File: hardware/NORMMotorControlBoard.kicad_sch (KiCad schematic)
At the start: 18 parts, among them J1 Back Left Motor, J2 Front Left Motor, J3 Front Right Motor, J4 Back Right Motor, J5 USB4125-GF-A_REVA2, J6 Conn_01x04_Pin, M1 Front Motors, M2 Back Motors, SW1 Reset, U1 SN74LVC2G14DBV, U2 SN74LVC2G14DBV

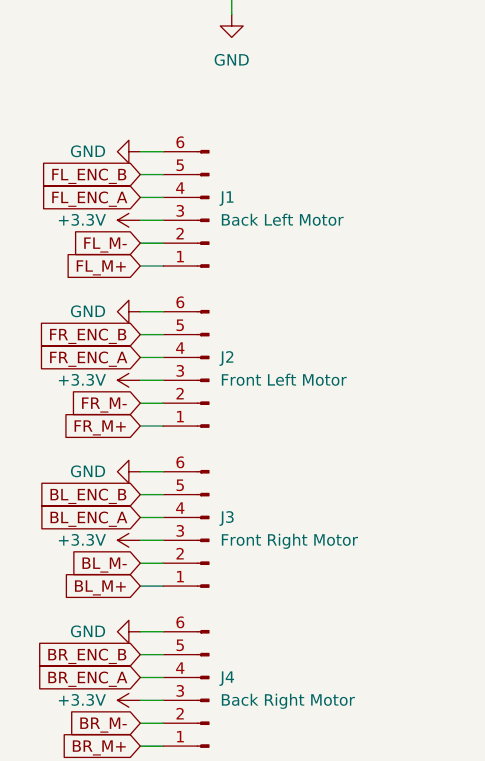
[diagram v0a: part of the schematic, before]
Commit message: Exported board v1.1
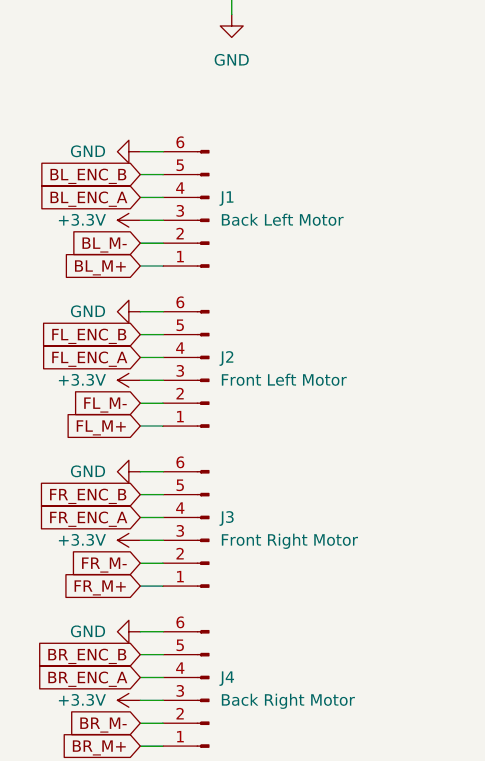
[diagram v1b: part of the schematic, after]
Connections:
- net BL_ENC_A: now also J1.4 (Pin_4); no longer J3.4 (Pin_4)
- net BL_ENC_B: now also J1.5 (Pin_5); no longer J3.5 (Pin_5)
- net BL_M+: now also J1.1 (Pin_1); no longer J3.1 (Pin_1)
- net BL_M-: now also J1.2 (Pin_2); no longer J3.2 (Pin_2)
- net FL_ENC_A: now also J2.4 (Pin_4); no longer J1.4 (Pin_4)
- net FL_ENC_B: now also J2.5 (Pin_5); no longer J1.5 (Pin_5)
- net FL_M+: now also J2.1 (Pin_1); no longer J1.1 (Pin_1)
- net FL_M-: now also J2.2 (Pin_2); no longer J1.2 (Pin_2)
- net FR_ENC_A: now also J3.4 (Pin_4); no longer J2.4 (Pin_4)
- net FR_ENC_B: now also J3.5 (Pin_5); no longer J2.5 (Pin_5)
- net FR_M+: now also J3.1 (Pin_1); no longer J2.1 (Pin_1)
- net FR_M-: now also J3.2 (Pin_2); no longer J2.2 (Pin_2)

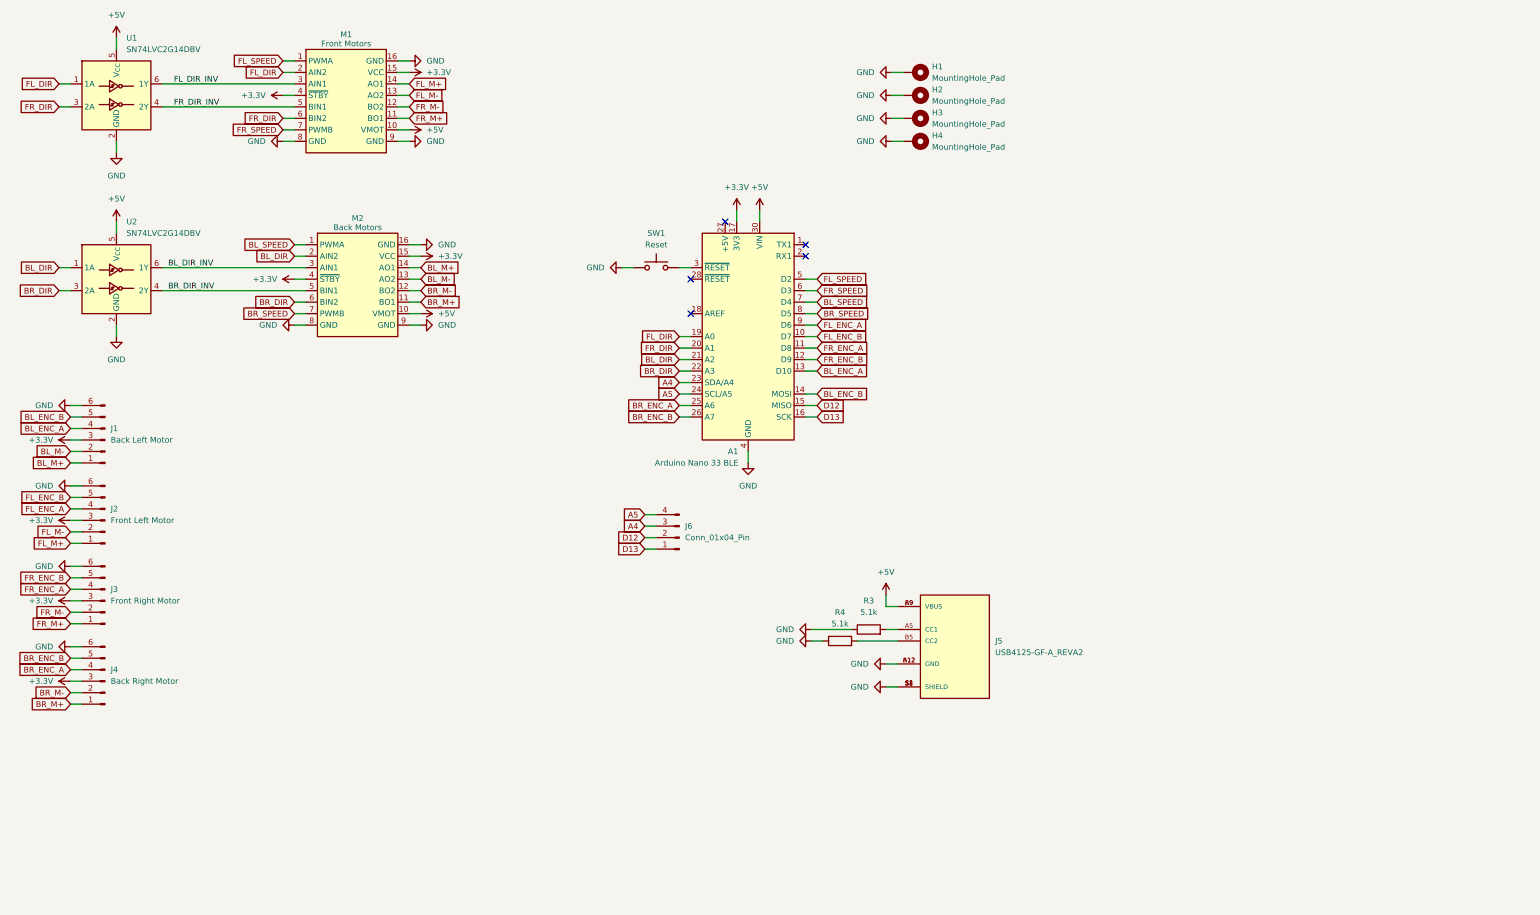
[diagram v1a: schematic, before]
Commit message: Finished schematic for V1.3
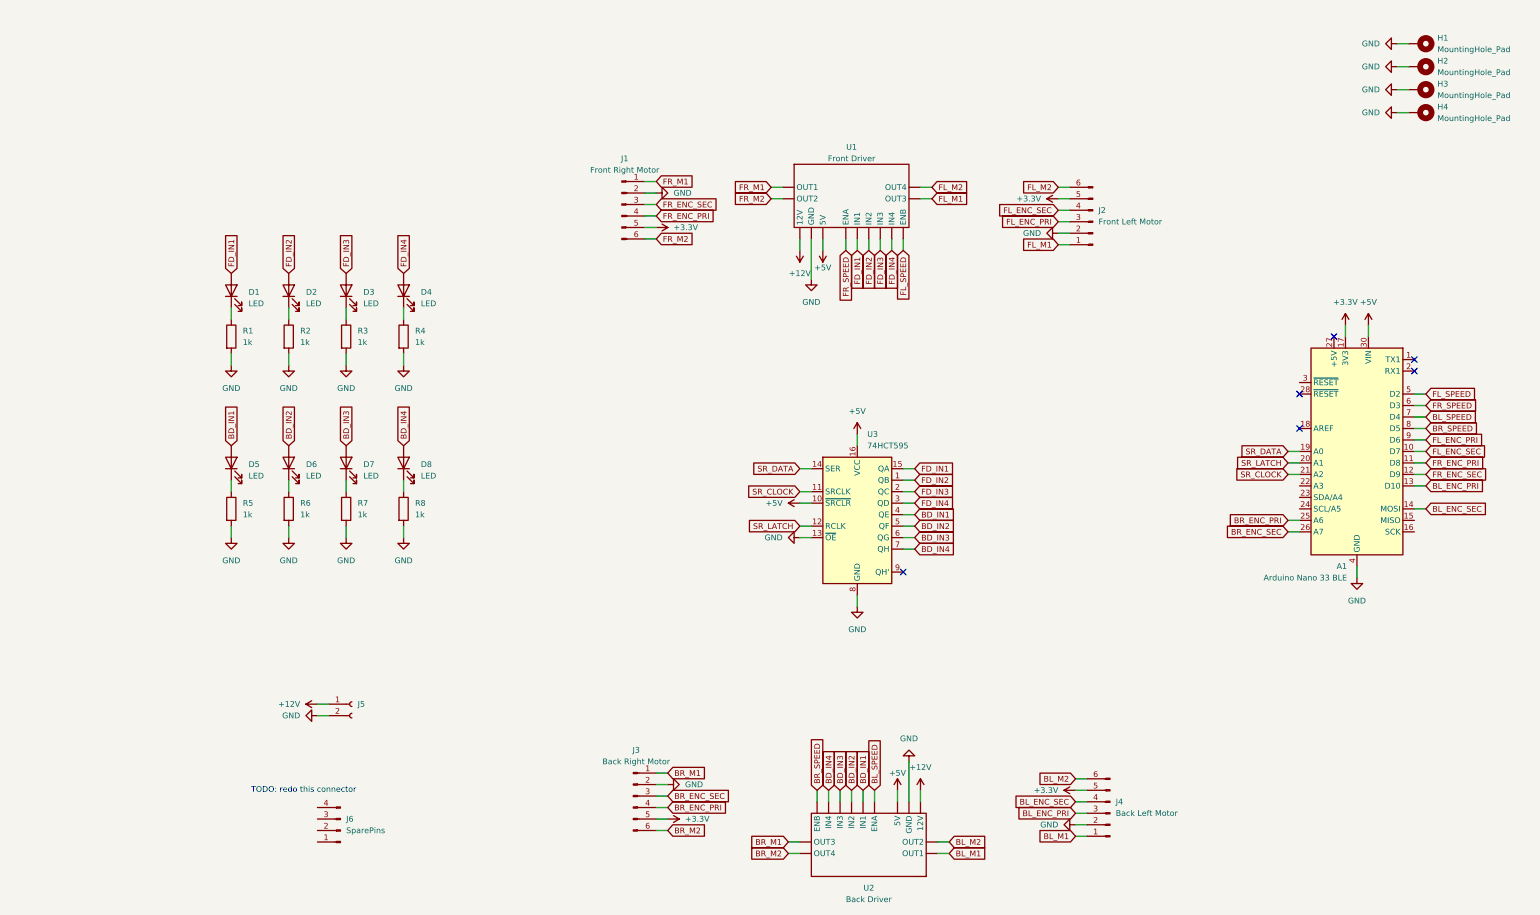
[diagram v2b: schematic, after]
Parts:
- removed J5: USB4125-GF-A_REVA2, USB_C:USB_C, symbol USB_C:USB4125-GF-A_REVA2
- removed M1: Front Motors, Pololu_MD08A_Motor_Driver:Pololu_MD08A_Motor_Driver, symbol Pololu_MD08A_Motor_Driver:Pololu_MD08A_Motor_Driver
- removed M2: Back Motors, Pololu_MD08A_Motor_Driver:Pololu_MD08A_Motor_Driver, symbol Pololu_MD08A_Motor_Driver:Pololu_MD08A_Motor_Driver
- removed SW1: Reset, Two_Pin_Through_Hole_Push_Button:Two_Pin_Through_Hole_Push_Button, symbol Switch:SW_Push
- removed U1, U2: SN74LVC2G14DBV, Package_TO_SOT_SMD:SOT-23-6, symbol 74xGxx:SN74LVC2G14DBV
- added D1, D2, D3, D4, D5, D6, D7, D8: LED, LED_SMD:LED_0603_1608Metric, symbol Device:LED
- added J5: Conn_01x02_Socket, Connector_Samtec_HPM_THT:Samtec_HPM-02-01-x-S_Straight_1x02_Pitch5.08mm, symbol Connector:Conn_01x02_Socket
- added R1, R2, R5, R6, R7, R8: 1k, Resistor_SMD:R_0603_1608Metric, symbol Device:R
- added U1: Front Driver, symbol L298N:L298N
- added U2: Back Driver, symbol L298N:L298N
- added U3: 74HCT595, Package_SO:SOIC-16_3.9x9.9mm_P1.27mm, symbol 74xx:74HCT595
- J1: value Back Left Motor -> Front Right Motor; footprint Connector_PinHeader_2.54mm:PinHeader_1x06_P2.54mm_Horizontal -> Connector_JST:JST_PH_S6B-PH-K_1x06_P2.00mm_Horizontal
- J2: footprint Connector_PinHeader_2.54mm:PinHeader_1x06_P2.54mm_Horizontal -> Connector_JST:JST_PH_S6B-PH-K_1x06_P2.00mm_Horizontal
- J3: value Front Right Motor -> Back Right Motor; footprint Connector_PinHeader_2.54mm:PinHeader_1x06_P2.54mm_Horizontal -> Connector_JST:JST_PH_S6B-PH-K_1x06_P2.00mm_Horizontal
- J4: value Back Right Motor -> Back Left Motor; footprint Connector_PinHeader_2.54mm:PinHeader_1x06_P2.54mm_Horizontal -> Connector_JST:JST_PH_S6B-PH-K_1x06_P2.00mm_Horizontal
- J6: value Conn_01x04_Pin -> SparePins
- R3, R4: value 5.1k -> 1k; footprint Resistor_SMD:R_0603_1608Metric_Pad0.98x0.95mm_HandSolder -> Resistor_SMD:R_0603_1608Metric
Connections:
- net BL_M- is gone; now on net GND: J1.2 (Pin_2)
- net BR_M- is gone; now on net GND: J4.2 (Pin_2)
- net FL_M- is gone; now on net GND: J2.2 (Pin_2)
- net FR_M- is gone; now on net GND: J3.2 (Pin_2)
- net +3.3V: now also J1.5 (Pin_5), J2.5 (Pin_5), J3.5 (Pin_5), J4.5 (Pin_5); no longer J1.3 (Pin_3), J2.3 (Pin_3), J3.3 (Pin_3), J4.3 (Pin_3)
- net +5V: now also U1. (OUT4), U2. (OUT4), U3.10 (~{SRCLR}), U3.16 (VCC)
- net BL_SPEED: now also U2. (OUT4)
- net BR_SPEED: now also U2. (OUT4)
- net FL_SPEED: now also U1. (OUT4)
- net FR_SPEED: now also U1. (OUT4)
- net GND: now also R3.2, R4.2, J5.2 (Pin_2), R1.2, R2.2, R5.2, R6.2, R7.2, R8.2, U1. (OUT4), U2. (OUT4), U3.13 (~{OE}), U3.8 (GND); no longer J1.6 (Pin_6), J2.6 (Pin_6), J3.6 (Pin_6), J4.6 (Pin_6), R3.1, R4.1
- net A4: no longer names the net of A1.23 (SDA/A4)
- net A4: no longer J6.3 (Pin_3)
- net A5: no longer names the net of A1.24 (SCL/A5)
- net A5: no longer J6.4 (Pin_4)
- net BL_DIR renamed SR_CLOCK
- net SR_CLOCK: now also U3.11 (SRCLK)
- net BL_ENC_A renamed BL_ENC_PRI
- net BL_ENC_PRI: now also J4.3 (Pin_3); no longer J1.4 (Pin_4)
- net BL_ENC_B renamed BL_ENC_SEC
- net BL_ENC_SEC: now also J4.4 (Pin_4); no longer J1.5 (Pin_5)
- net BL_M+ renamed FR_M1
- net FR_M1: now also U1. (OUT4)
- net BR_DIR: no longer names the net of A1.22 (A3)
- net BR_ENC_A renamed BR_ENC_PRI
- net BR_ENC_PRI: now also J3.4 (Pin_4); no longer J4.4 (Pin_4)
- net BR_ENC_B renamed BR_ENC_SEC
- net BR_ENC_SEC: now also J3.3 (Pin_3); no longer J4.5 (Pin_5)
- net BR_M+ renamed BL_M1
- net BL_M1: now also U2. (OUT4)
- net D12: no longer names the net of A1.15 (MISO)
- net D12: no longer J6.2 (Pin_2)
- net D13: no longer names the net of A1.16 (SCK)
- net D13: no longer J6.1 (Pin_1)
- net FL_DIR renamed SR_DATA
- net SR_DATA: now also U3.14 (SER)
- net FL_ENC_A renamed FL_ENC_PRI
- net FL_ENC_PRI: now also J2.3 (Pin_3); no longer J2.4 (Pin_4)
- net FL_ENC_B renamed FL_ENC_SEC
- net FL_ENC_SEC: now also J2.4 (Pin_4); no longer J2.5 (Pin_5)
- net FL_M+ renamed FL_M1
- net FL_M1: now also U1. (OUT4)
- net FR_DIR renamed SR_LATCH
- net SR_LATCH: now also U3.12 (RCLK)
- net FR_ENC_A renamed FR_ENC_PRI
- net FR_ENC_PRI: now also J1.4 (Pin_4); no longer J3.4 (Pin_4)
- net FR_ENC_B renamed FR_ENC_SEC
- net FR_ENC_SEC: now also J1.3 (Pin_3); no longer J3.5 (Pin_5)
- net FR_M+ renamed BR_M1
- net BR_M1: now also U2. (OUT4)
- new net: D6.1 (K), R6.1
- new net: D4.1 (K), R4.1
- new net: D3.1 (K), R3.1
- new net: D2.1 (K), R2.1
- new net: D7.1 (K), R7.1
- new net: D5.1 (K), R5.1
- new net: D1.1 (K), R1.1
- new net: D8.1 (K), R8.1
- new net +12V: J5.1 (Pin_1), U1. (OUT4), U2. (OUT4)
- new net BD_IN1: D5.2 (A), U2. (OUT4), U3.4 (QE)
- new net BD_IN2: D6.2 (A), U2. (OUT4), U3.5 (QF)
- new net BD_IN3: D7.2 (A), U2. (OUT4), U3.6 (QG)
- new net BD_IN4: D8.2 (A), U2. (OUT4), U3.7 (QH)
- new net BL_M2: J4.6 (Pin_6), U2. (OUT4)
- new net BR_M2: J3.6 (Pin_6), U2. (OUT4)
- new net FD_IN1: D1.2 (A), U1. (OUT4), U3.15 (QA)
- new net FD_IN2: D2.2 (A), U1. (OUT4), U3.1 (QB)
- new net FD_IN3: D3.2 (A), U1. (OUT4), U3.2 (QC)
- new net FD_IN4: D4.2 (A), U1. (OUT4), U3.3 (QD)
- new net FL_M2: J2.6 (Pin_6), U1. (OUT4)
- new net FR_M2: J1.6 (Pin_6), U1. (OUT4)
- no-connect marks 5 -> 6
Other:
- note added: "TODO: redo this connector"
- moved on the sheet: A1, H1, H2, H3, H4, J6

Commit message: Finished schematic for V1.2
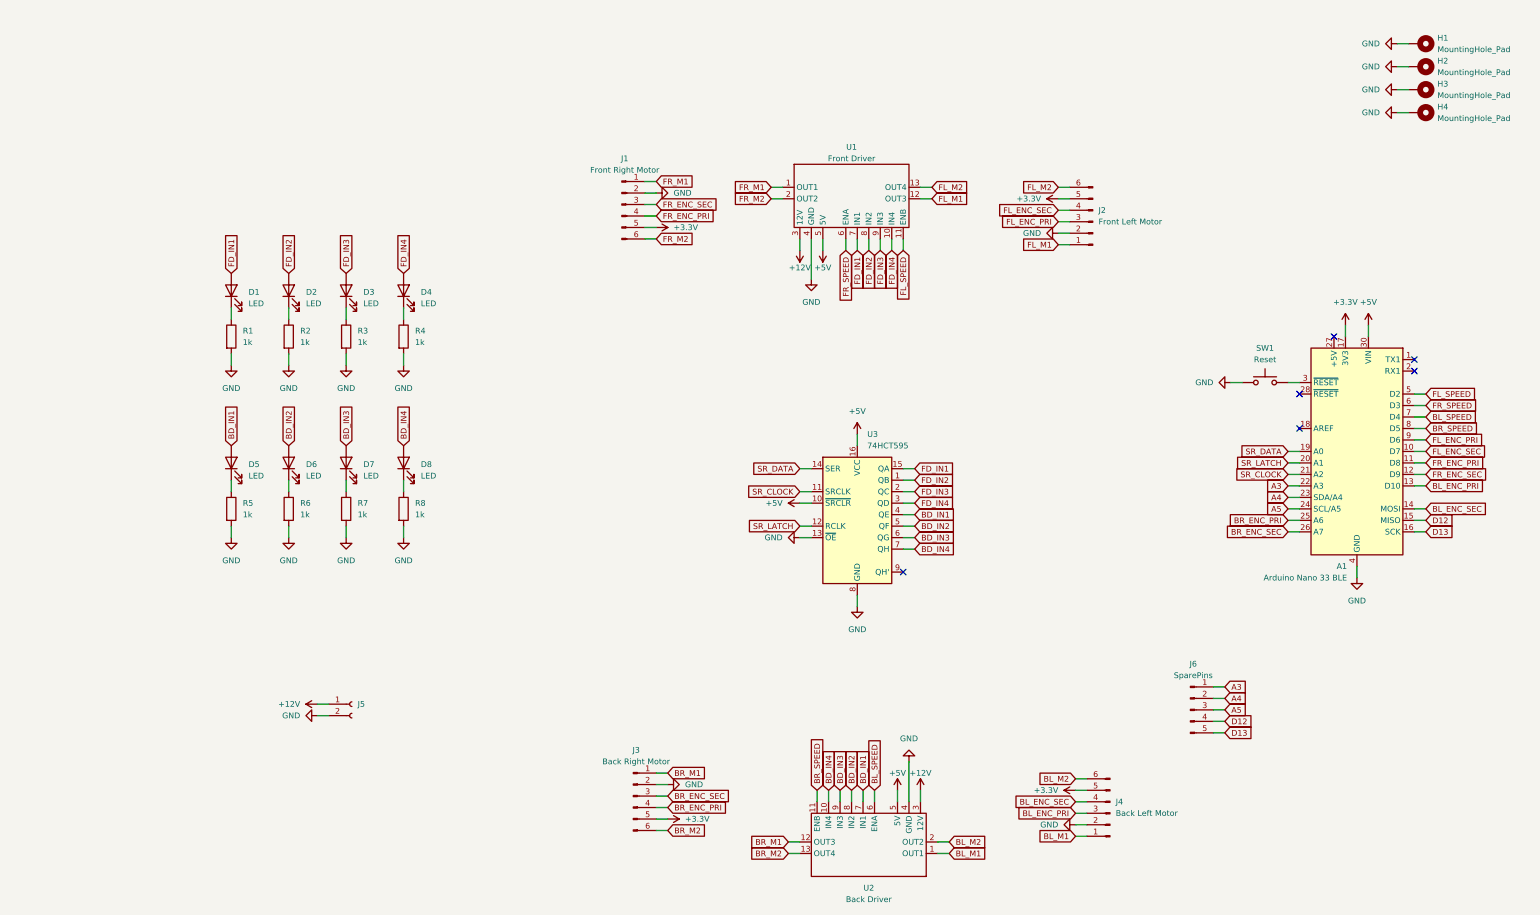
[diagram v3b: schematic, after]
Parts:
- added SW1: Reset, Two_Pin_Through_Hole_Push_Button:Two_Pin_Through_Hole_Push_Button, symbol Switch:SW_Push
- J6: footprint Connector_PinHeader_2.54mm:PinHeader_1x04_P2.54mm_Vertical -> Connector_PinHeader_2.54mm:PinHeader_1x05_P2.54mm_Vertical; symbol Connector:Conn_01x04_Pin -> Connector:Conn_01x05_Pin
- U1, U2: footprint (none) -> L298N:L298N
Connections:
- net +12V: now also U1.3 (12V), U2.3 (12V); no longer U1. (OUT4), U2. (OUT4)
- net +5V: now also U1.5 (5V), U2.5 (5V); no longer U1. (OUT4), U2. (OUT4)
- net BD_IN1: now also U2.7 (IN1); no longer U2. (OUT4)
- net BD_IN2: now also U2.8 (IN2); no longer U2. (OUT4)
- net BD_IN3: now also U2.9 (IN3); no longer U2. (OUT4)
- net BD_IN4: now also U2.10 (IN4); no longer U2. (OUT4)
- net BL_M1: now also U2.1 (OUT1); no longer U2. (OUT4)
- net BL_M2: now also U2.2 (OUT2); no longer U2. (OUT4)
- net BL_SPEED: now also U2.6 (ENA); no longer U2. (OUT4)
- net BR_M1: now also U2.12 (OUT3); no longer U2. (OUT4)
- net BR_M2: now also U2.13 (OUT4); no longer U2. (OUT4)
- net BR_SPEED: now also U2.11 (ENB); no longer U2. (OUT4)
- net FD_IN1: now also U1.7 (IN1); no longer U1. (OUT4)
- net FD_IN2: now also U1.8 (IN2); no longer U1. (OUT4)
- net FD_IN3: now also U1.9 (IN3); no longer U1. (OUT4)
- net FD_IN4: now also U1.10 (IN4); no longer U1. (OUT4)
- net FL_M1: now also U1.12 (OUT3); no longer U1. (OUT4)
- net FL_M2: now also U1.13 (OUT4); no longer U1. (OUT4)
- net FL_SPEED: now also U1.11 (ENB); no longer U1. (OUT4)
- net FR_M1: now also U1.1 (OUT1); no longer U1. (OUT4)
- net FR_M2: now also U1.2 (OUT2); no longer U1. (OUT4)
- net FR_SPEED: now also U1.6 (ENA); no longer U1. (OUT4)
- net GND: now also U1.4 (GND), U2.4 (GND), SW1.1; no longer U1. (OUT4), U2. (OUT4)
- net D12: now reaches A1.15 (MISO)
- net D12: now also J6.4 (Pin_4)
- net D13: now reaches A1.16 (SCK)
- net D13: now also J6.5 (Pin_5)
- net A3: now reaches A1.22 (A3)
- net A3: now also J6.1 (Pin_1)
- net A4: now reaches A1.23 (SDA/A4)
- net A4: now also J6.2 (Pin_2)
- net A5: now reaches A1.24 (SCL/A5)
- net A5: now also J6.3 (Pin_3)
- net at A1.3 (~{RESET}): now also SW1.2
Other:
- note removed: "TODO: redo this connector"
